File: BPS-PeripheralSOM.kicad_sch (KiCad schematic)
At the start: 20 parts, among them J2 Can_In, J7 SWD, SW2 Reset, U1 STM32L431CBTx, Y1 8M

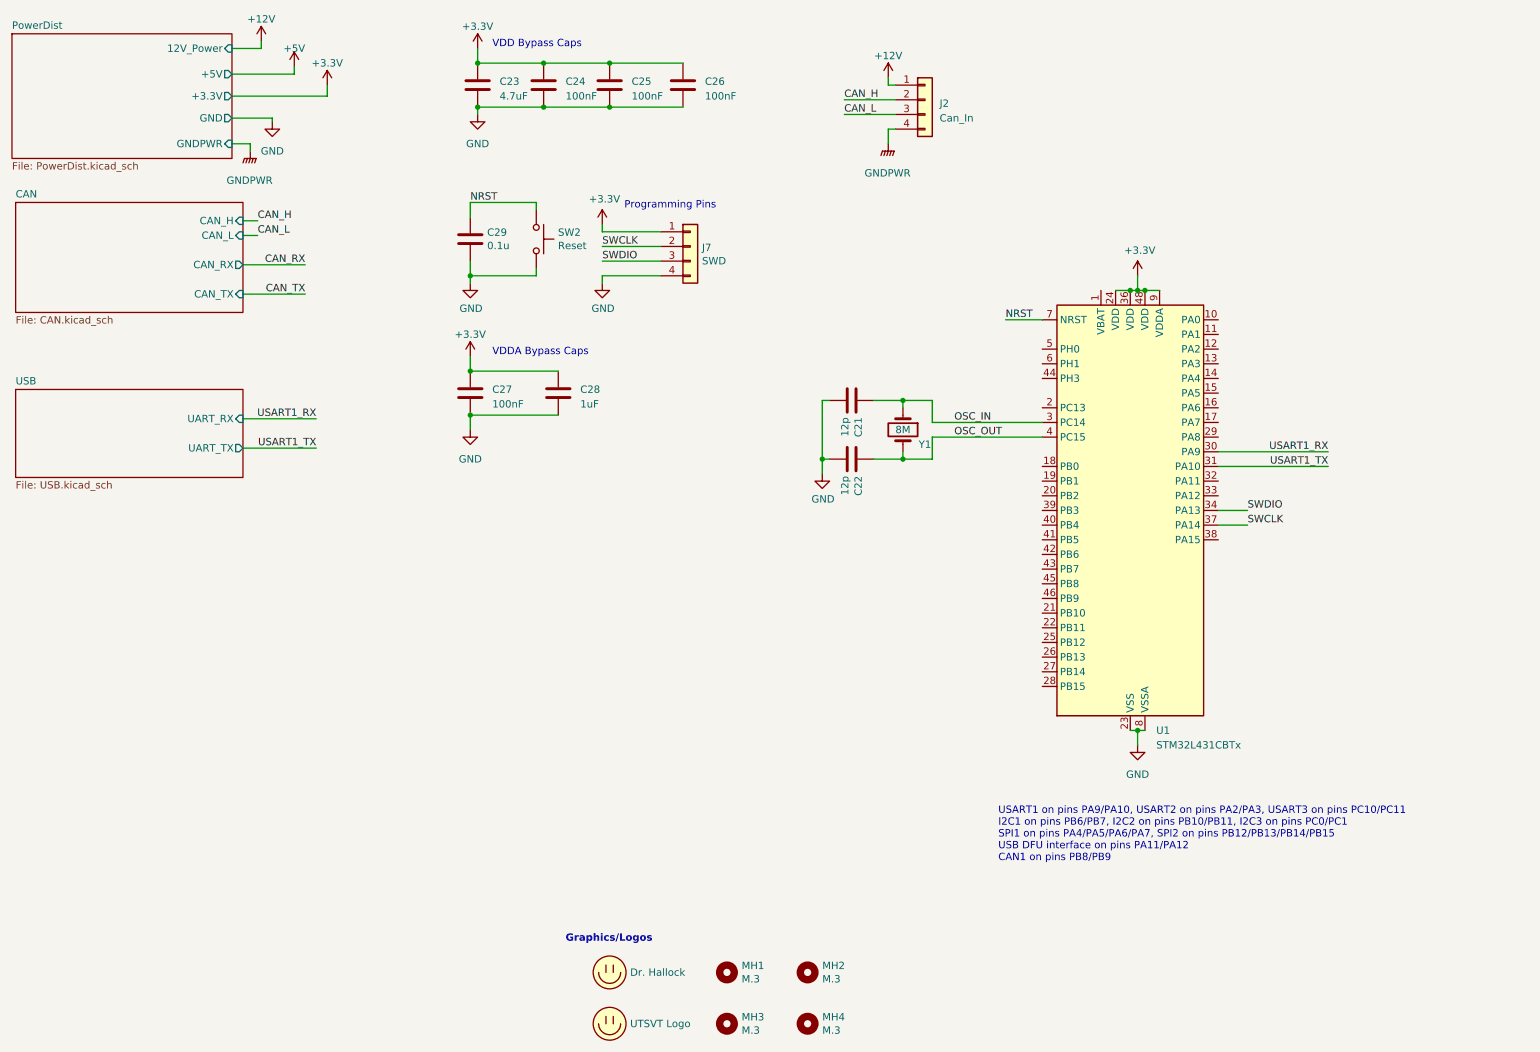
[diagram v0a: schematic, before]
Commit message: you kiss your mom with that face?
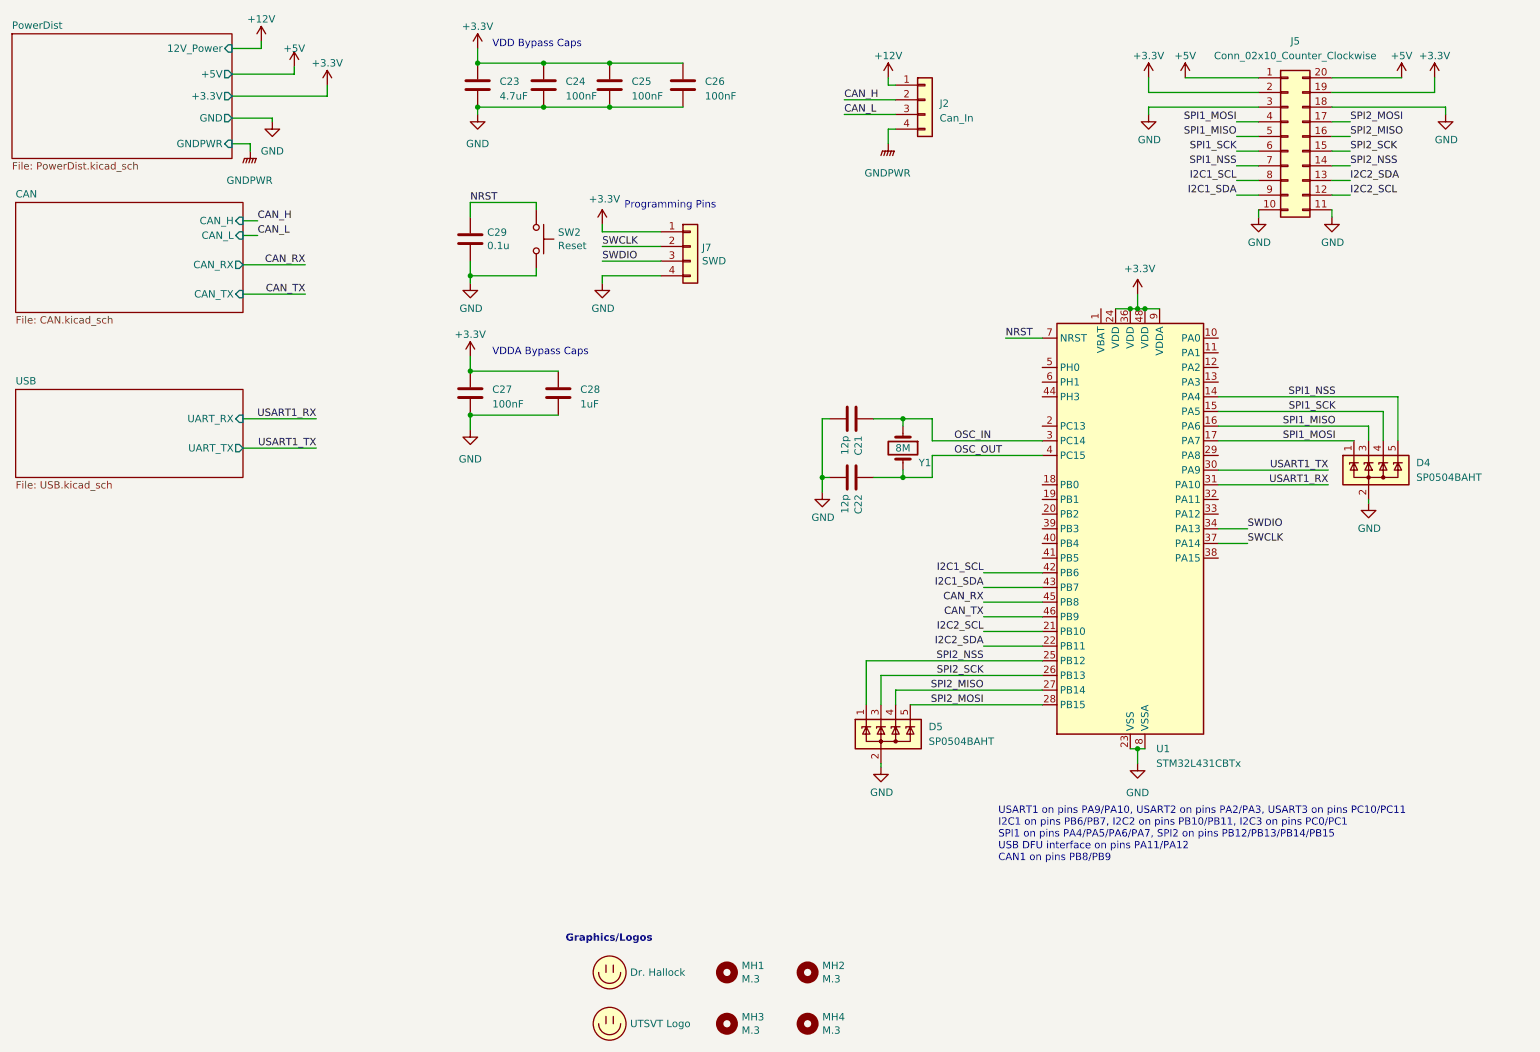
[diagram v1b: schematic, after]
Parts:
- added D4, D5: SP0504BAHT, Package_TO_SOT_SMD:SOT-23-5, symbol Power_Protection:SP0504BAHT
- added J5: Conn_02x10_Counter_Clockwise, symbol Connector_Generic:Conn_02x10_Counter_Clockwise
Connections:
- net +3.3V: now also J5.19 (Pin_19), J5.2 (Pin_2)
- net +5V: now also J5.1 (Pin_1), J5.20 (Pin_20)
- net CAN_RX: now also U1.45 (PB8)
- net CAN_TX: now also U1.46 (PB9)
- net GND: now also D4.2 (A), D5.2 (A), J5.10 (Pin_10), J5.11 (Pin_11), J5.18 (Pin_18), J5.3 (Pin_3)
- net USART1_RX: now also U1.31 (PA10); no longer U1.30 (PA9)
- net USART1_TX: now also U1.30 (PA9); no longer U1.31 (PA10)
- net SPI1_NSS: now reaches U1.14 (PA4)
- net SPI1_NSS: now also D4.5 (K), J5.7 (Pin_7)
- net SPI1_SCK: now reaches U1.15 (PA5)
- net SPI1_SCK: now also D4.4 (K), J5.6 (Pin_6)
- net SPI1_MISO: now reaches U1.16 (PA6)
- net SPI1_MISO: now also D4.3 (K), J5.5 (Pin_5)
- net SPI1_MOSI: now reaches U1.17 (PA7)
- net SPI1_MOSI: now also D4.1 (K), J5.4 (Pin_4)
- net I2C2_SCL: now reaches U1.21 (PB10)
- net I2C2_SCL: now also J5.12 (Pin_12)
- net I2C2_SDA: now reaches U1.22 (PB11)
- net I2C2_SDA: now also J5.13 (Pin_13)
- net SPI2_NSS: now reaches U1.25 (PB12)
- net SPI2_NSS: now also D5.1 (K), J5.14 (Pin_14)
- net SPI2_SCK: now reaches U1.26 (PB13)
- net SPI2_SCK: now also D5.3 (K), J5.15 (Pin_15)
- net SPI2_MISO: now reaches U1.27 (PB14)
- net SPI2_MISO: now also D5.4 (K), J5.16 (Pin_16)
- net SPI2_MOSI: now reaches U1.28 (PB15)
- net SPI2_MOSI: now also D5.5 (K), J5.17 (Pin_17)
- net I2C1_SCL: now reaches U1.42 (PB6)
- net I2C1_SCL: now also J5.8 (Pin_8)
- net I2C1_SDA: now reaches U1.43 (PB7)
- net I2C1_SDA: now also J5.9 (Pin_9)
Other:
- moved on the sheet: C21, C22, U1, Y1
